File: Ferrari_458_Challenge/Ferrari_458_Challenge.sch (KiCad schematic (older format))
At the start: 30 parts, among them P1 SERVO, P2 ESC, P3 LEFT_IR, P4 RIGHT_IR, P5 ULTRASONIC, P6 7.4V_BATTERY, P7 12V_BATTERY, Q3 2N3904, Q4 FQP47P06, U1 LM7805, U2 FS-R6B, U3 Arduino_mega

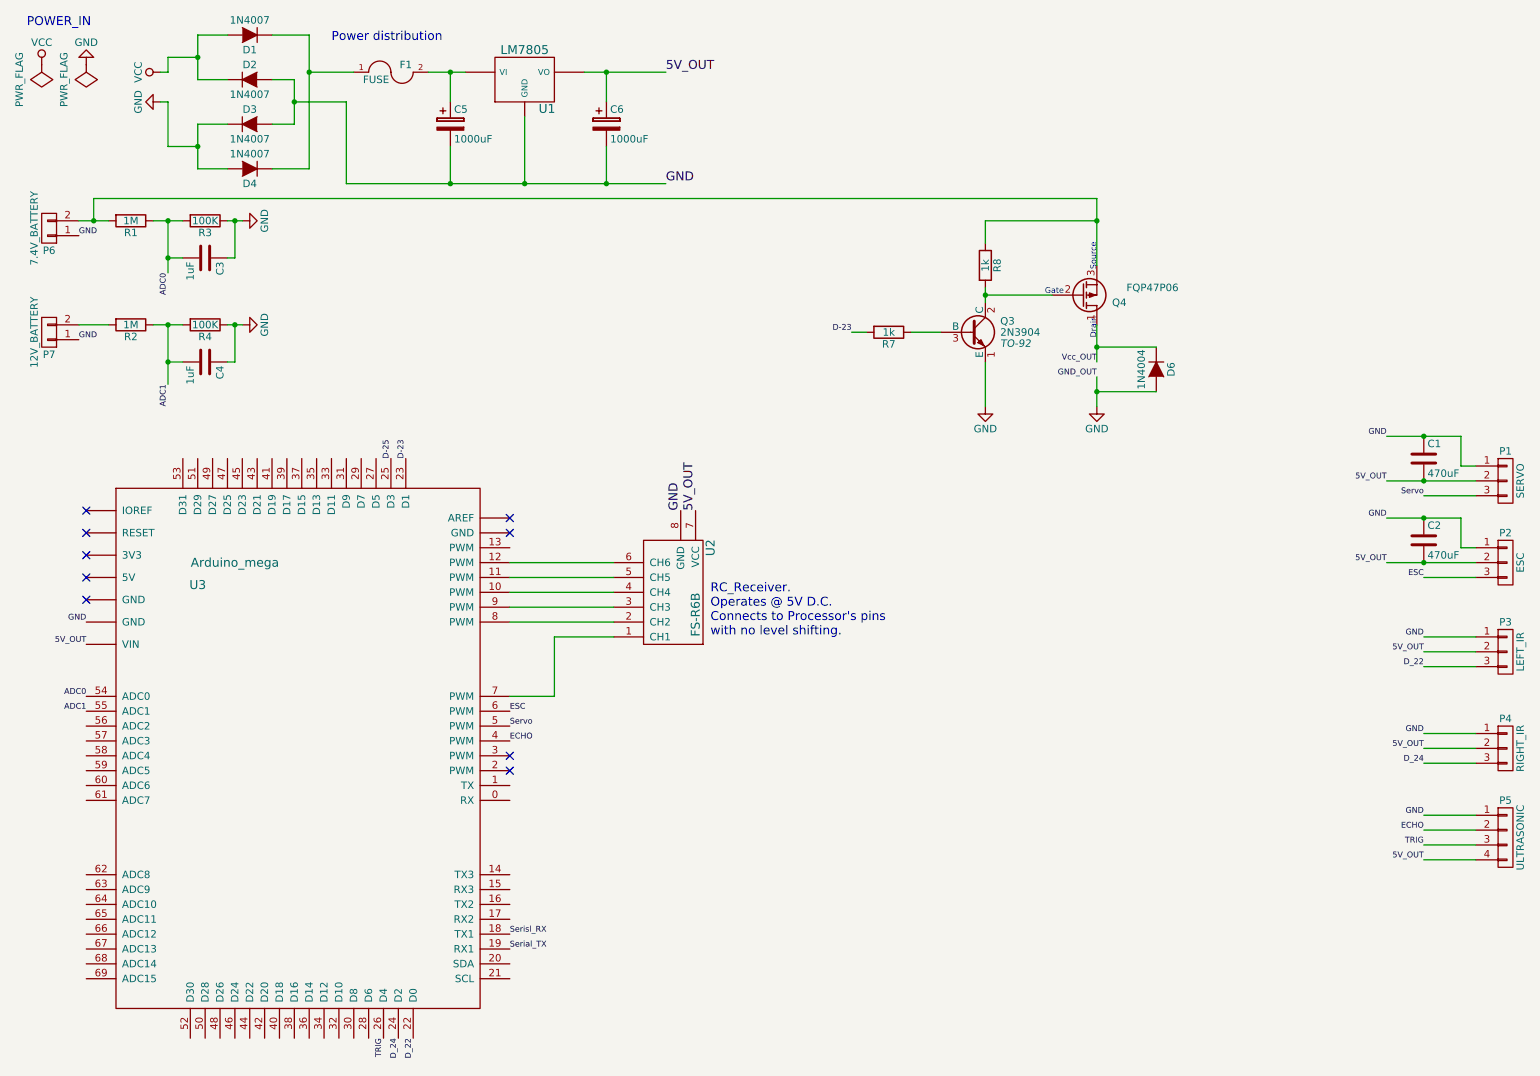
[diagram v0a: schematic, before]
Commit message: Schematic update
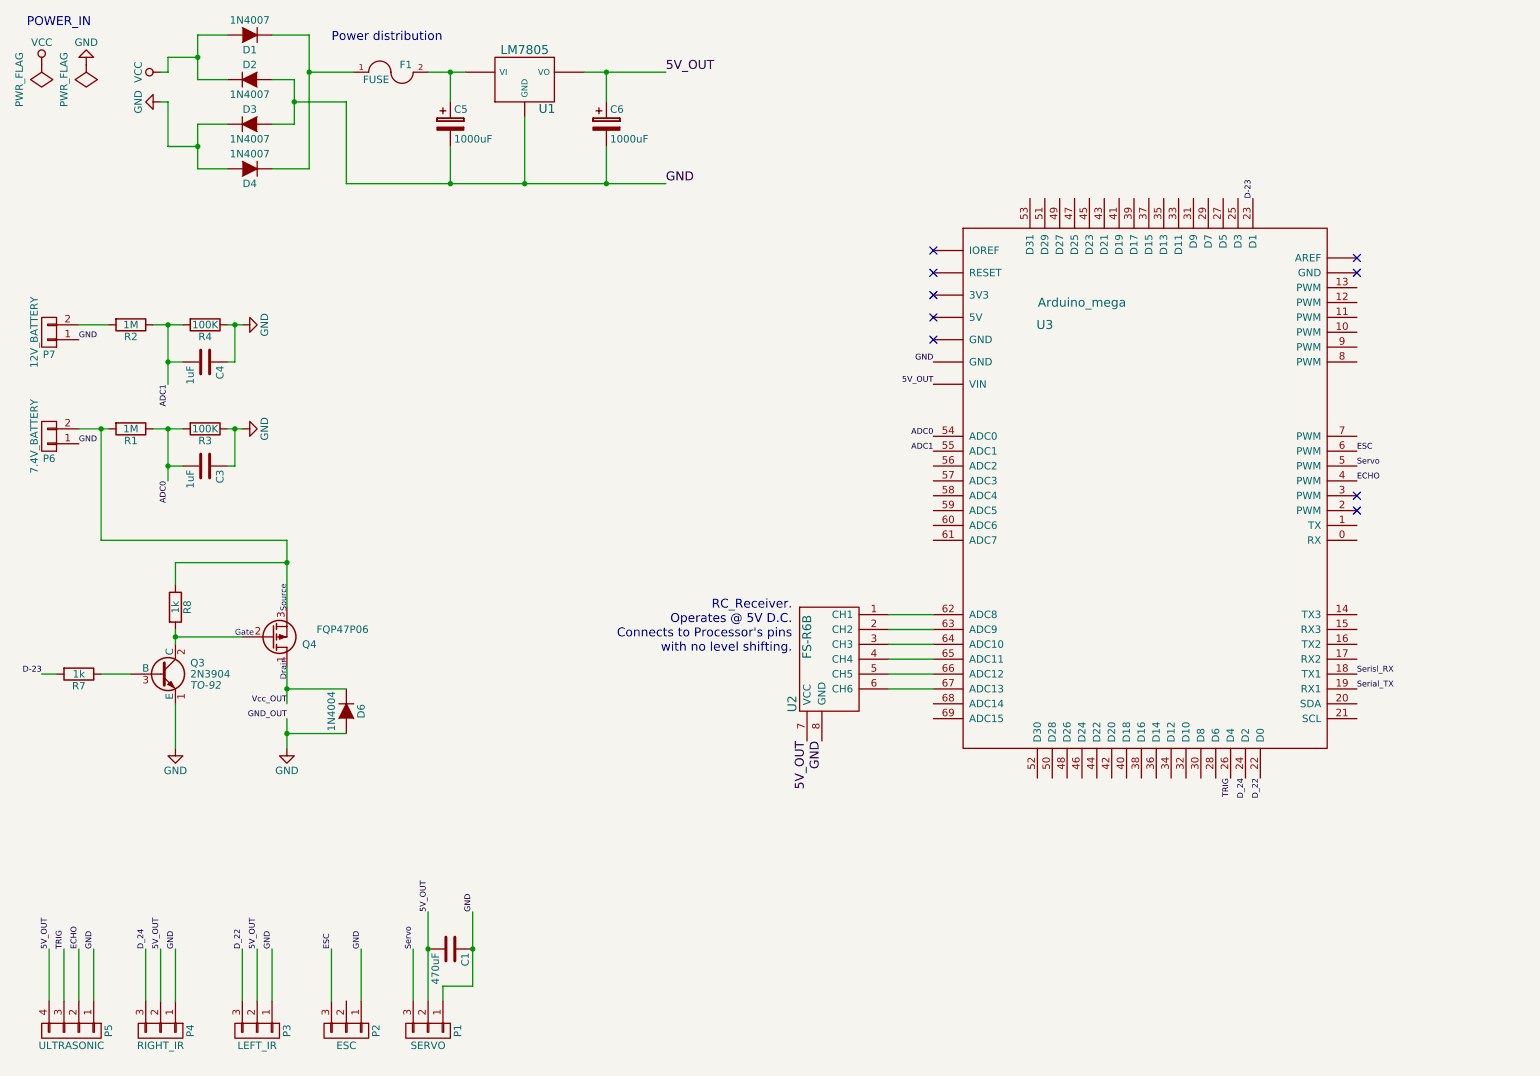
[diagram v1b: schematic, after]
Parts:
- removed C2: 470uF, symbol C
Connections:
- net 5V_OUT: no longer P2.2 (P2)
- net at U2.1 (CH1): now also U3.62 (ADC8); no longer U3.7 (PWM)
- net at U2.2 (CH2): now also U3.63 (ADC9); no longer U3.8 (PWM)
- net at U2.3 (CH3): now also U3.64 (ADC10); no longer U3.9 (PWM)
- net at U2.4 (CH4): now also U3.65 (ADC11); no longer U3.10 (PWM)
- net at U2.5 (CH5): now also U3.66 (ADC12); no longer U3.11 (PWM)
- net at U2.6 (CH6): now also U3.67 (ADC13); no longer U3.12 (PWM)
- net D-25: no longer names the net of U3.25 (D3)
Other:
- moved on the sheet: C1, C3, D6, P1, P2, P3, P4, P5, P6, Q3, Q4, R1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
